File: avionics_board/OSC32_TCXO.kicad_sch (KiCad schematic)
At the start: 2 parts, among them X3 32.768KHZ

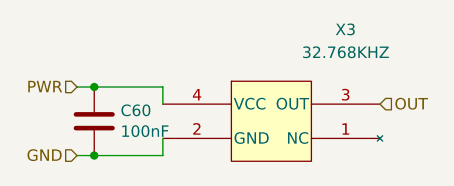
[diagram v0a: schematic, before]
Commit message: VRef+ meeds to be connected to VDDA, should not be left floating
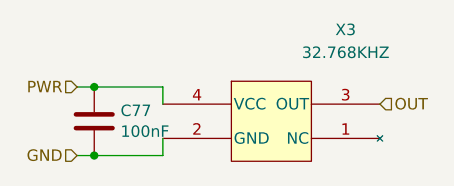
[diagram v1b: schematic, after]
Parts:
- renumbered C60 to C77
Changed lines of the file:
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@@
 		(on_board yes)
 		(dnp no)
-		(property "Reference" "C60"
+		(property "Reference" "C77"
 			(at 132.461 122.6566 0)
 			(effects
@@
 			(project "sci_board"
 				(path "/b4b2c88d-f6cd-4e60-862d-e21f68728580/840799ac-4fe6-4a8e-96a2-299affeec8e4/9565b29f-739e-499d-a066-98bd4c80d38b"
-					(reference "C60")
+					(reference "C77")
 					(unit 1)
 				)

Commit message: SCI bodge board to correct I2C switching
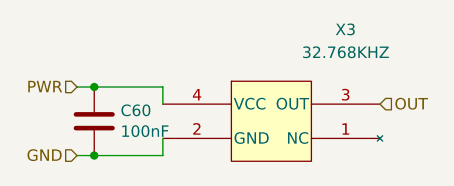
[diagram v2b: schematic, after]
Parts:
- renumbered C77 to C60
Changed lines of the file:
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@@
 		(on_board yes)
 		(dnp no)
-		(property "Reference" "C77"
+		(property "Reference" "C60"
 			(at 132.461 122.6566 0)
 			(effects
@@
 			(project "sci_board"
 				(path "/b4b2c88d-f6cd-4e60-862d-e21f68728580/840799ac-4fe6-4a8e-96a2-299affeec8e4/9565b29f-739e-499d-a066-98bd4c80d38b"
-					(reference "C77")
+					(reference "C60")
 					(unit 1)
 				)
